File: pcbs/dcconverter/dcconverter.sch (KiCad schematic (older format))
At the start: 44 parts, among them IC1 NCP7805TG, J1 190-9991, J3 146-8335, J4 766-6604, J5 766-6604, Q1 NGTB40N120FL2WG, Q10 TS13003CT, Q2 FQP47P06, Q3 2SK3747-1E, Q4 2SK3747-1E, Q5 TS13003CT, Q6 TS13003CT, Q7 FQP3P50, Q8 FDP20N50

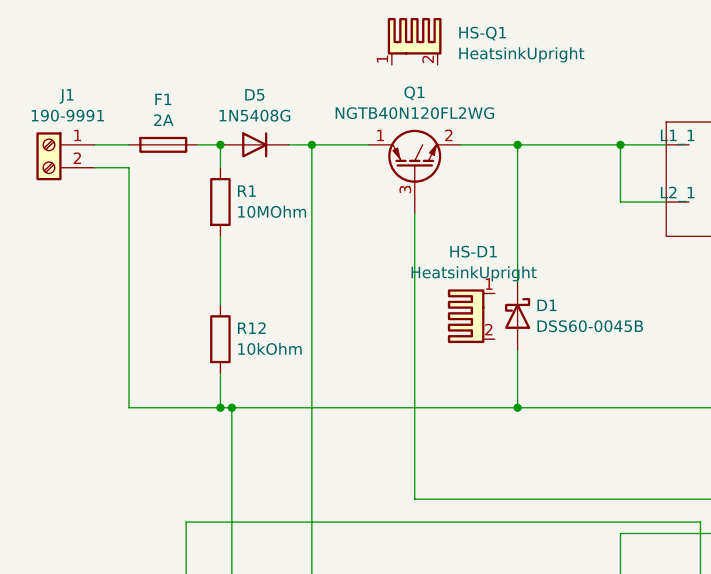
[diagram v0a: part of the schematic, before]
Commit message: Fix minor stuff
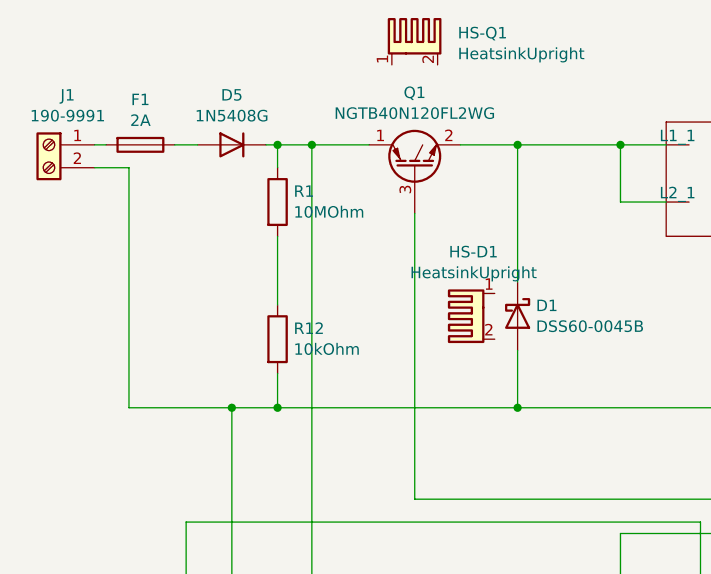
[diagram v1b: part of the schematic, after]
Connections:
- net at D5.1 (K), Q1.1 (C), Q3.3 (D)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: now also R1.1
- net at D5.2 (A), F1.1: no longer R1.1
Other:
- moved on the sheet: D5, F1, R1, R12
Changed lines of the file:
@@
 L Device:Fuse F1
 U 1 1 5F93C935
-P 1350 1950
-F 0 "F1" V 1153 1950 50  0000 C CNN
-F 1 "2A" V 1244 1950 50  0000 C CNN
-F 2 "Fuse:Fuseholder_Cylinder-5x20mm_Schurter_0031_8201_Horizontal_Open" V 1280 1950 50  0001 C CNN
-F 3 "~" H 1350 1950 50  0001 C CNN
-	1    1350 1950
-	0    1    1    0
-$EndComp
-Wire Wire Line
-	1050 1950 1200 1950
+P 1250 1950
+F 0 "F1" V 1053 1950 50  0000 C CNN
+F 1 "2A" V 1144 1950 50  0000 C CNN
+F 2 "Fuse:Fuseholder_Cylinder-5x20mm_Schurter_0031_8201_Horizontal_Open" V 1180 1950 50  0001 C CNN
+F 3 "~" H 1250 1950 50  0001 C CNN
+	1    1250 1950
+	0    1    1    0
+$EndComp
 $Comp
 L Device:D_Schottky D1
@@
 L Device:D D5
 U 1 1 5FBA5BAB
-P 1750 1950
-F 0 "D5" H 1750 2167 50  0000 C CNN
-F 1 "1N5408G" H 1750 2076 50  0000 C CNN
-F 2 "Custom:1N5408G" H 1750 1950 50  0001 C CNN
-F 3 "~" H 1750 1950 50  0001 C CNN
-	1    1750 1950
+P 1650 1950
+F 0 "D5" H 1650 2167 50  0000 C CNN
+F 1 "1N5408G" H 1650 2076 50  0000 C CNN
+F 2 "Custom:1N5408G" H 1650 1950 50  0001 C CNN
+F 3 "~" H 1650 1950 50  0001 C CNN
+	1    1650 1950
 	-1   0    0    -1
 $EndComp
-Wire Wire Line
-	1500 1950 1600 1950
-Wire Wire Line
-	1900 1950 2000 1950
 Connection ~ 2000 1950
 Wire Wire Line
-	1650 3100 2900 3100
+	1650 3100 1850 3100
 $Comp
 L Device:R R1
 U 1 1 5FBBC80C
-P 1600 2200
-F 0 "R1" H 1670 2246 50  0000 L CNN
-F 1 "10MOhm" H 1670 2155 50  0000 L CNN
-F 2 "Resistor_THT:R_Axial_DIN0207_L6.3mm_D2.5mm_P10.16mm_Horizontal" V 1530 2200 50  0001 C CNN
-F 3 "~" H 1600 2200 50  0001 C CNN
-	1    1600 2200
+P 1850 2200
+F 0 "R1" H 1920 2246 50  0000 L CNN
+F 1 "10MOhm" H 1920 2155 50  0000 L CNN
+F 2 "Resistor_THT:R_Axial_DIN0207_L6.3mm_D2.5mm_P10.16mm_Horizontal" V 1780 2200 50  0001 C CNN
+F 3 "~" H 1850 2200 50  0001 C CNN
+	1    1850 2200
 	1    0    0    -1
 $EndComp
@@
 L Device:R R12
 U 1 1 5FBBD1DD
-P 1600 2800
-F 0 "R12" H 1670 2846 50  0000 L CNN
-F 1 "10kOhm" H 1670 2755 50  0000 L CNN
-F 2 "Resistor_THT:R_Axial_DIN0207_L6.3mm_D2.5mm_P10.16mm_Horizontal" V 1530 2800 50  0001 C CNN
-F 3 "~" H 1600 2800 50  0001 C CNN
-	1    1600 2800
-	1    0    0    -1
-$EndComp
-Wire Wire Line
-	1600 1950 1600 2050
-Connection ~ 1600 1950
-Wire Wire Line
-	1600 2350 1600 2650
-Wire Wire Line
-	1600 2950 1600 3100
-Wire Wire Line
-	1600 3100 1650 3100
+P 1850 2800
+F 0 "R12" H 1920 2846 50  0000 L CNN
+F 1 "10kOhm" H 1920 2755 50  0000 L CNN
+F 2 "Resistor_THT:R_Axial_DIN0207_L6.3mm_D2.5mm_P10.16mm_Horizontal" V 1780 2800 50  0001 C CNN
+F 3 "~" H 1850 2800 50  0001 C CNN
+	1    1850 2800
+	1    0    0    -1
+$EndComp
+Wire Wire Line
+	1850 2350 1850 2650
 Connection ~ 1650 3100
 Wire Wire Line
-	1600 3100 1200 3100
-Wire Wire Line
 	1200 3100 1200 2050
 Wire Wire Line
 	1200 2050 1050 2050
-Connection ~ 1600 3100
+Wire Wire Line
+	1200 3100 1650 3100
+Wire Wire Line
+	1050 1950 1100 1950
+Wire Wire Line
+	1400 1950 1500 1950
+Wire Wire Line
+	1800 1950 1850 1950
+Wire Wire Line
+	1850 2050 1850 1950
+Connection ~ 1850 1950
+Wire Wire Line
+	1850 1950 2000 1950
+Wire Wire Line
+	1850 2950 1850 3100
+Connection ~ 1850 3100
+Wire Wire Line
+	1850 3100 2900 3100
 $EndSCHEMATC
